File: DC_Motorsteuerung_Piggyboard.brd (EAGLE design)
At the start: 35.2 x 100 mm, 16 parts

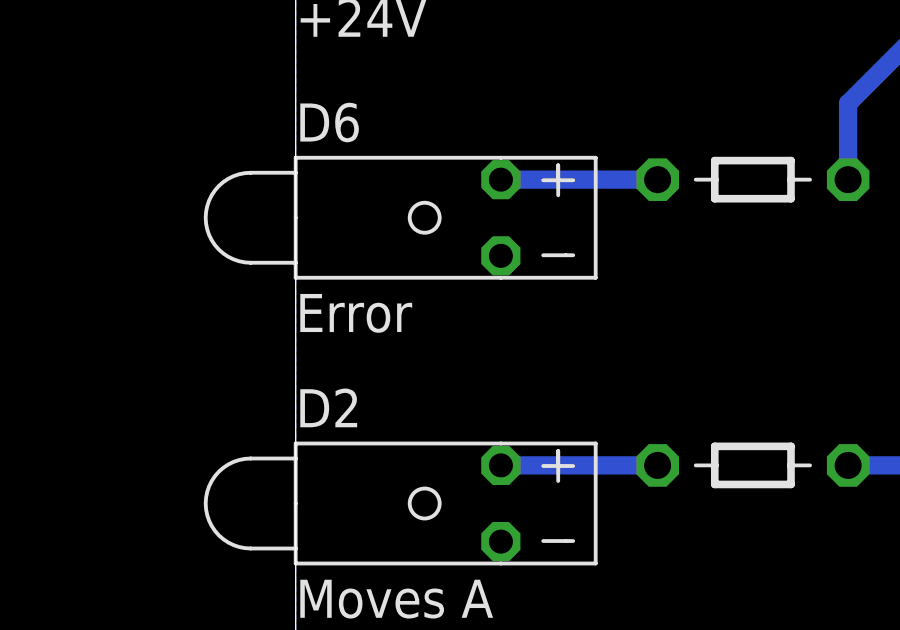
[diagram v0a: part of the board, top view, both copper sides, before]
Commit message: Piggiboard updated
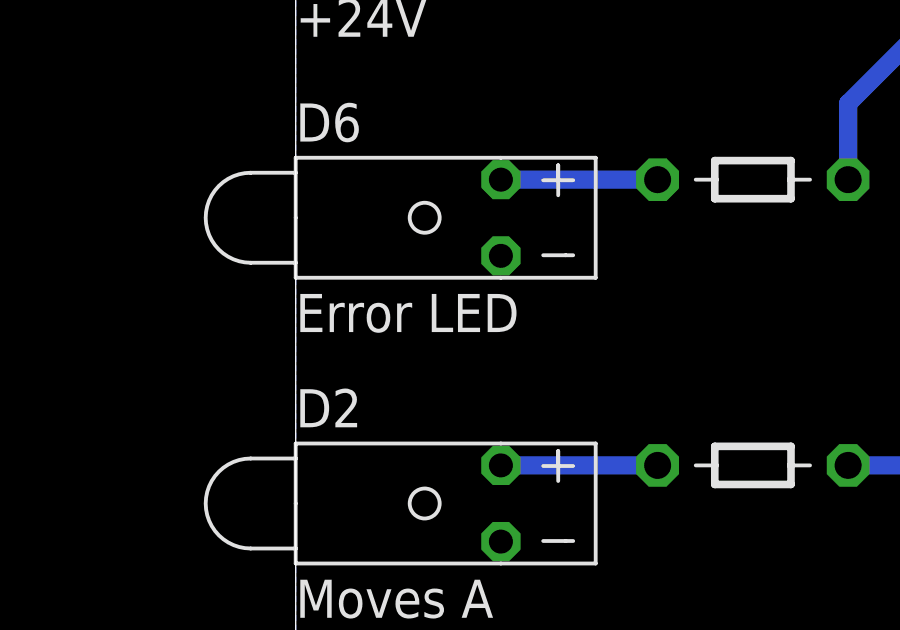
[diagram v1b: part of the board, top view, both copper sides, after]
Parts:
- D6: value Error -> Error LED
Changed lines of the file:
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@@
 <attribute name="VALUE" x="19.05" y="48.5775" size="1.778" layer="27" rot="R180"/>
 </element>
-<element name="D6" library="Test" package="LED3MMCASE" value="Error" x="0" y="43.815"/>
+<element name="D6" library="Test" package="LED3MMCASE" value="Error LED" x="0" y="43.815"/>
 </elements>
 <signals>

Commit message: Piggiboard updated
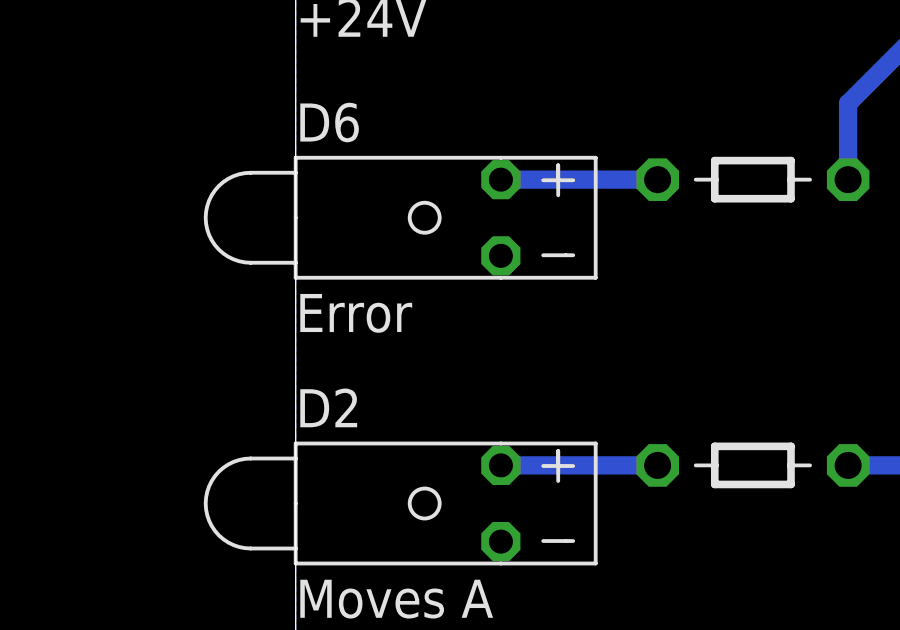
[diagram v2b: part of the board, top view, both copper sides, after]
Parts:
- D6: value Error LED -> Error
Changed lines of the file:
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@@
 <attribute name="VALUE" x="19.05" y="48.5775" size="1.778" layer="27" rot="R180"/>
 </element>
-<element name="D6" library="Test" package="LED3MMCASE" value="Error LED" x="0" y="43.815"/>
+<element name="D6" library="Test" package="LED3MMCASE" value="Error" x="0" y="43.815"/>
 </elements>
 <signals>
